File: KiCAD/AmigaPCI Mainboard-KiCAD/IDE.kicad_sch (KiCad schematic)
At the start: 43 parts, among them CN20 SECONDARY IDE, CN227 JTAG/SWD, CN5 PRIMARY IDE, CN6 IDE_LED, J202 SYSTEM CLK, J905 CABLE SELECT, U2 XC9572XL-VQ64, U220 74AHCT08, U900 74HCT245, U901 74HCT245, U902 74HCT245, U904 74HCT245, U905 74FCT646, U906 74FCT646

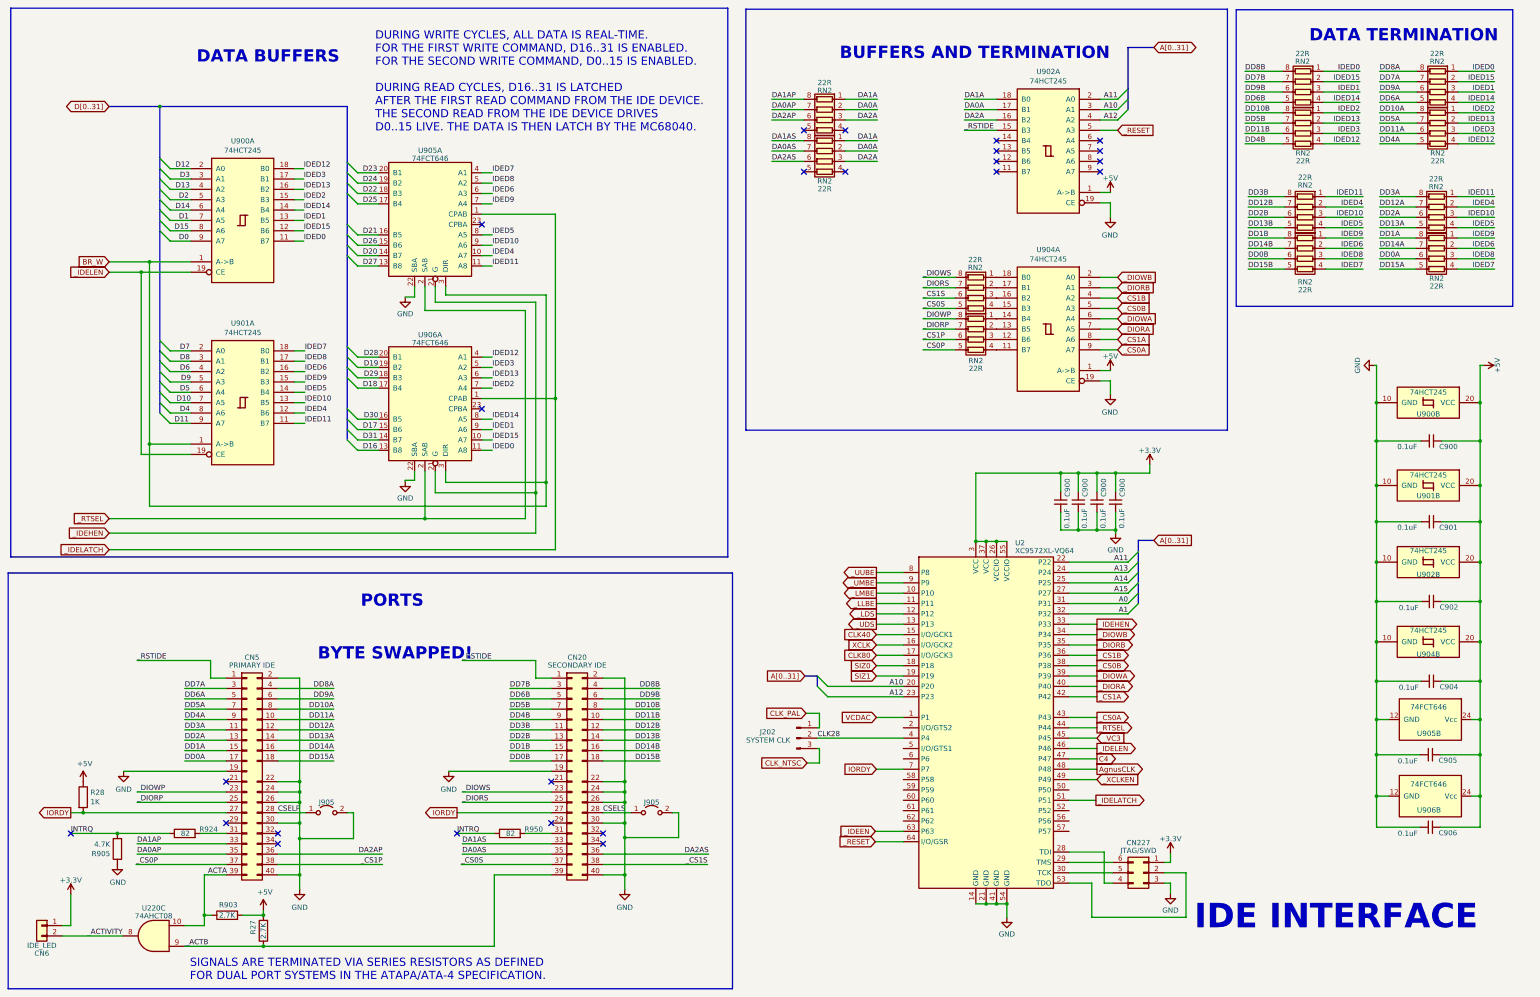
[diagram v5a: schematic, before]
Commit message: Routing 23-DEC-2023
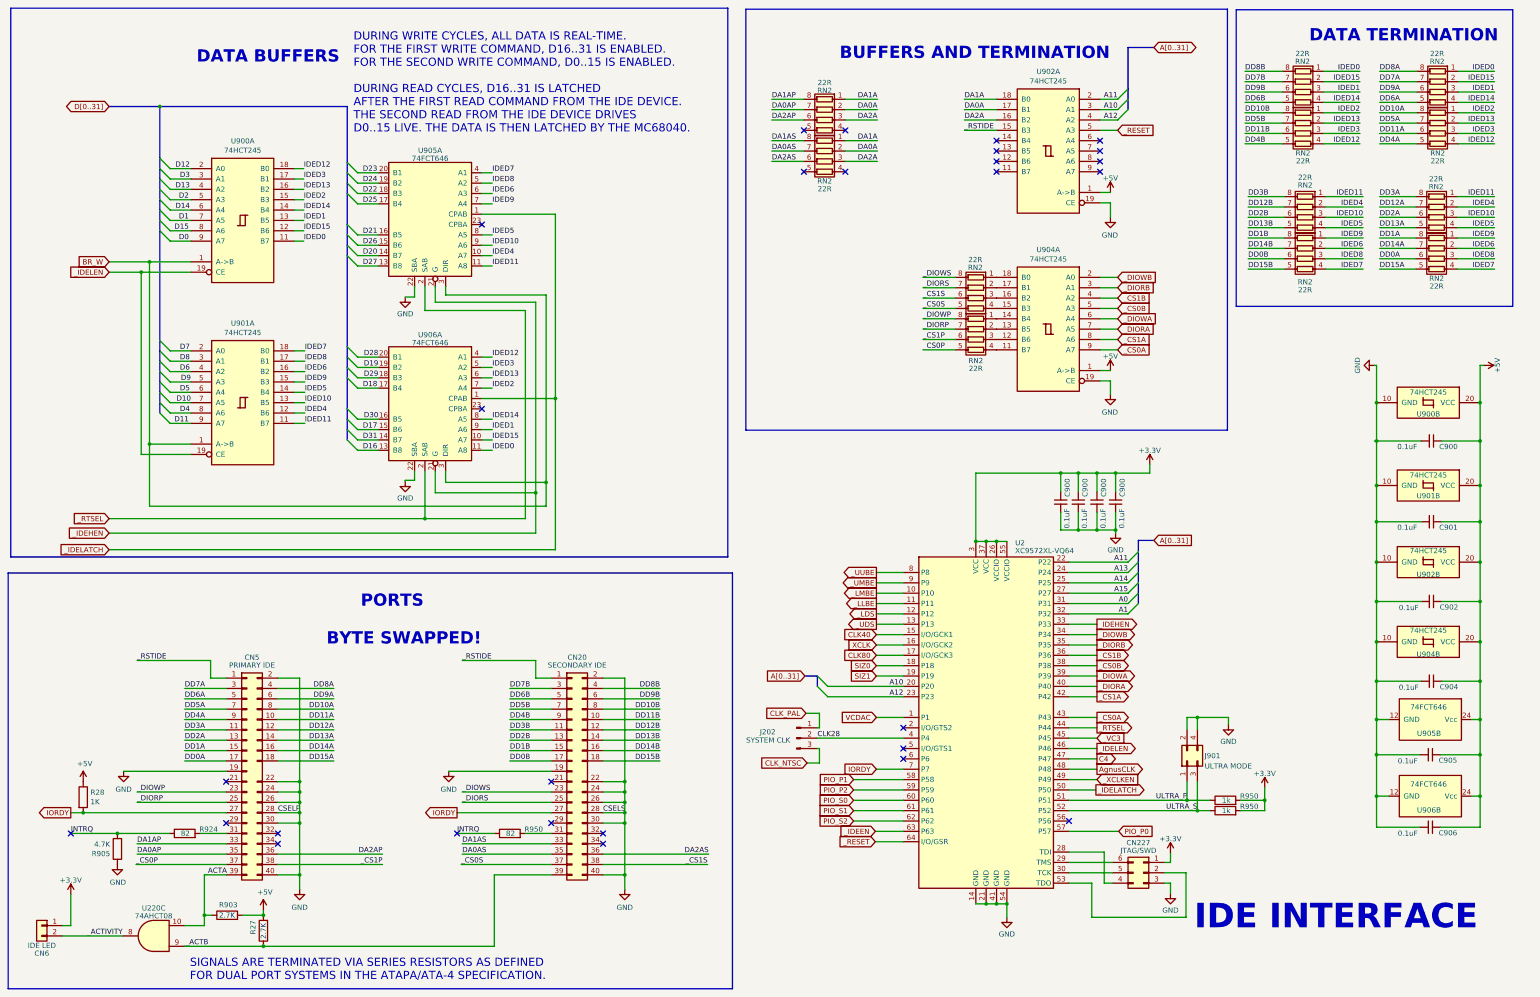
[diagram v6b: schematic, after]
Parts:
- removed J905 (x2): CABLE SELECT, Connector_PinHeader_2.54mm:PinHeader_1x02_P2.54mm_Vertical, symbol Jumper:Jumper_2_Open
- added J901: ULTRA MODE, Connector_PinHeader_2.54mm:PinHeader_2x02_P2.54mm_Vertical, symbol Connector_Generic:Conn_02x02_Odd_Even
- added R950 (x2): 1k, Resistor_SMD:R_0603_1608Metric, symbol Device:R
- CN6: value IDE_LED -> IDE LED
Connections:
- net CSELP is gone; now on net GND: CN5.28 (Pin_28)
- net CSELS is gone; now on net GND: CN20.28 (Pin_28)
- net +3.3V: now also R950.2, R950.2
- net GND: now also J901.2 (Pin_2), J901.4 (Pin_4)
- net _IDELATCH: now also U2.50 (P50); no longer U2.51 (P51)
- net ULTRA_S: now reaches U2.52 (P52)
- net ULTRA_S: now also J901.3 (Pin_3), R950.1
- net PIO_P0: now reaches U2.57 (P57)
- net PIO_P1: now reaches U2.58 (P58)
- net PIO_P2: now reaches U2.59 (P59)
- net PIO_S0: now reaches U2.60 (P60)
- net PIO_S1: now reaches U2.61 (P61)
- net PIO_S2: now reaches U2.62 (P62)
- new net ULTRA_P: J901.1 (Pin_1), R950.1, U2.51 (P51)
- no-connect marks 24 -> 28
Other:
- note added: "DURING WRITE CYCLES, ALL DATA IS REAL-TIME. FOR THE FIRST WRITE COMMAND, D16..31 IS ENABLED. FOR THE SECOND WRITE COMMAND, D0..15 IS ENABLED. DURING READ CYCLES, D16..31 IS LATCHED AFTER THE FIRST READ COMMAND FROM THE IDE DEVICE. THE SECOND READ FROM THE IDE DEVICE DRIVES D0..15 LIVE. THE DATA IS THEN LATCHED BY THE MC68040."
- note removed: "DURING WRITE CYCLES, ALL DATA IS REAL-TIME. FOR THE FIRST WRITE COMMAND, D16..31 IS ENABLED. FOR THE SECOND WRITE COMMAND, D0..15 IS ENABLED. DURING READ CYCLES, D16..31 IS LATCHED AFTER THE FIRST READ COMMAND FROM THE IDE DEVICE. THE SECOND READ FROM THE IDE DEVICE DRIVES D0..15 LIVE. THE DATA IS THEN LATCH BY THE MC68040."
